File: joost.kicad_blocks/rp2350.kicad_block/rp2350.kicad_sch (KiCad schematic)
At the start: 44 parts, among them U1 GT-USB-7010ASV, U2 RP2350_80QFN, U3 W25Q128, U4 APS6404L-3SQR-SN_C5333729, Y1 ABM8-272-T3

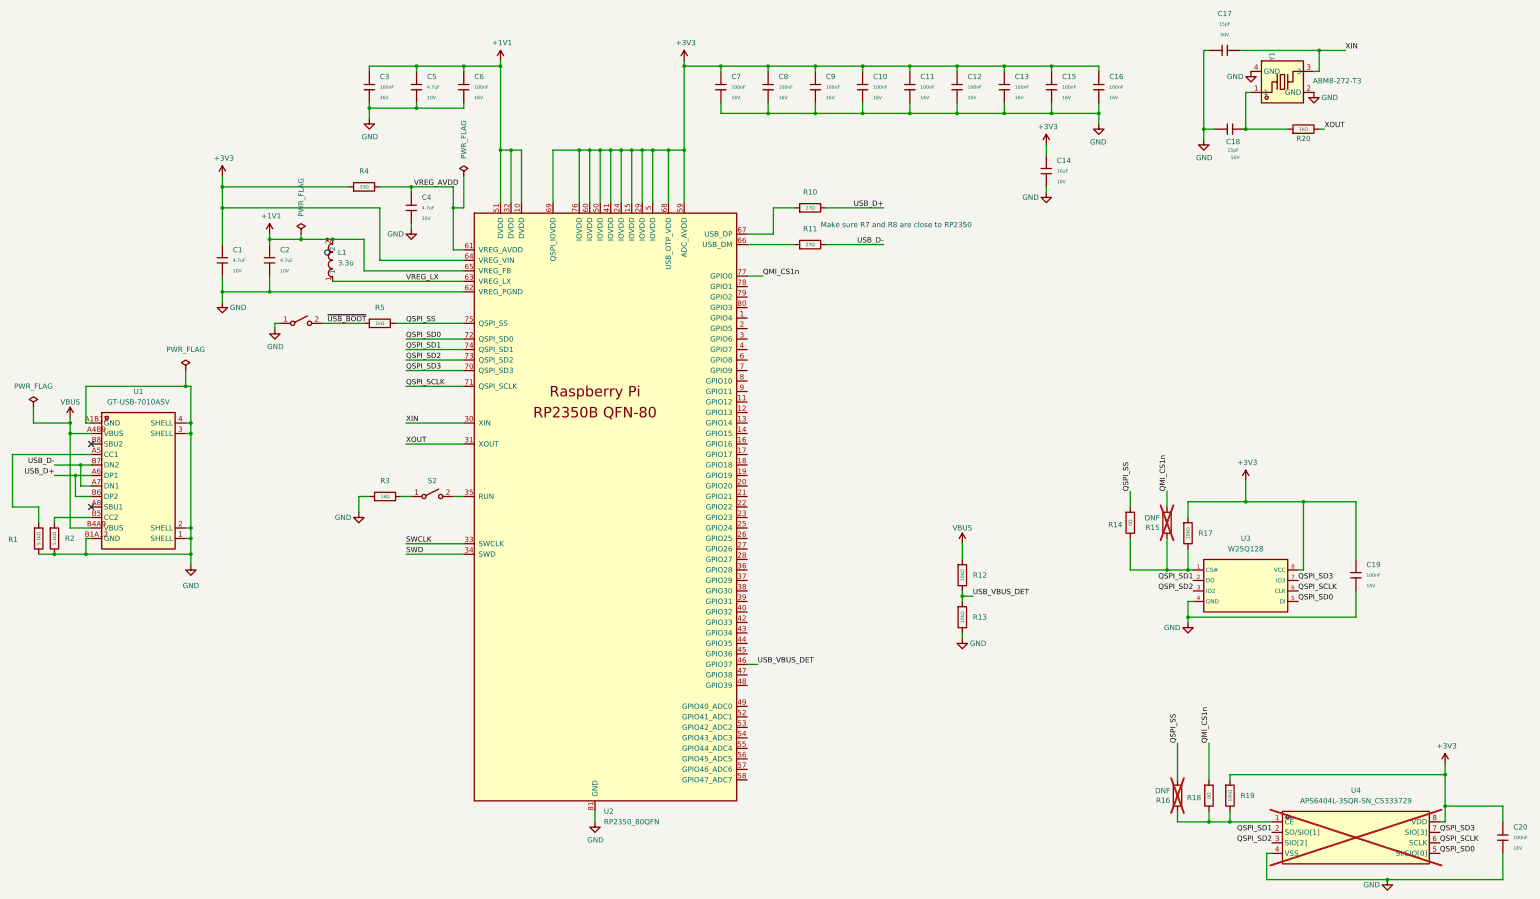
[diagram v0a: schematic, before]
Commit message: -
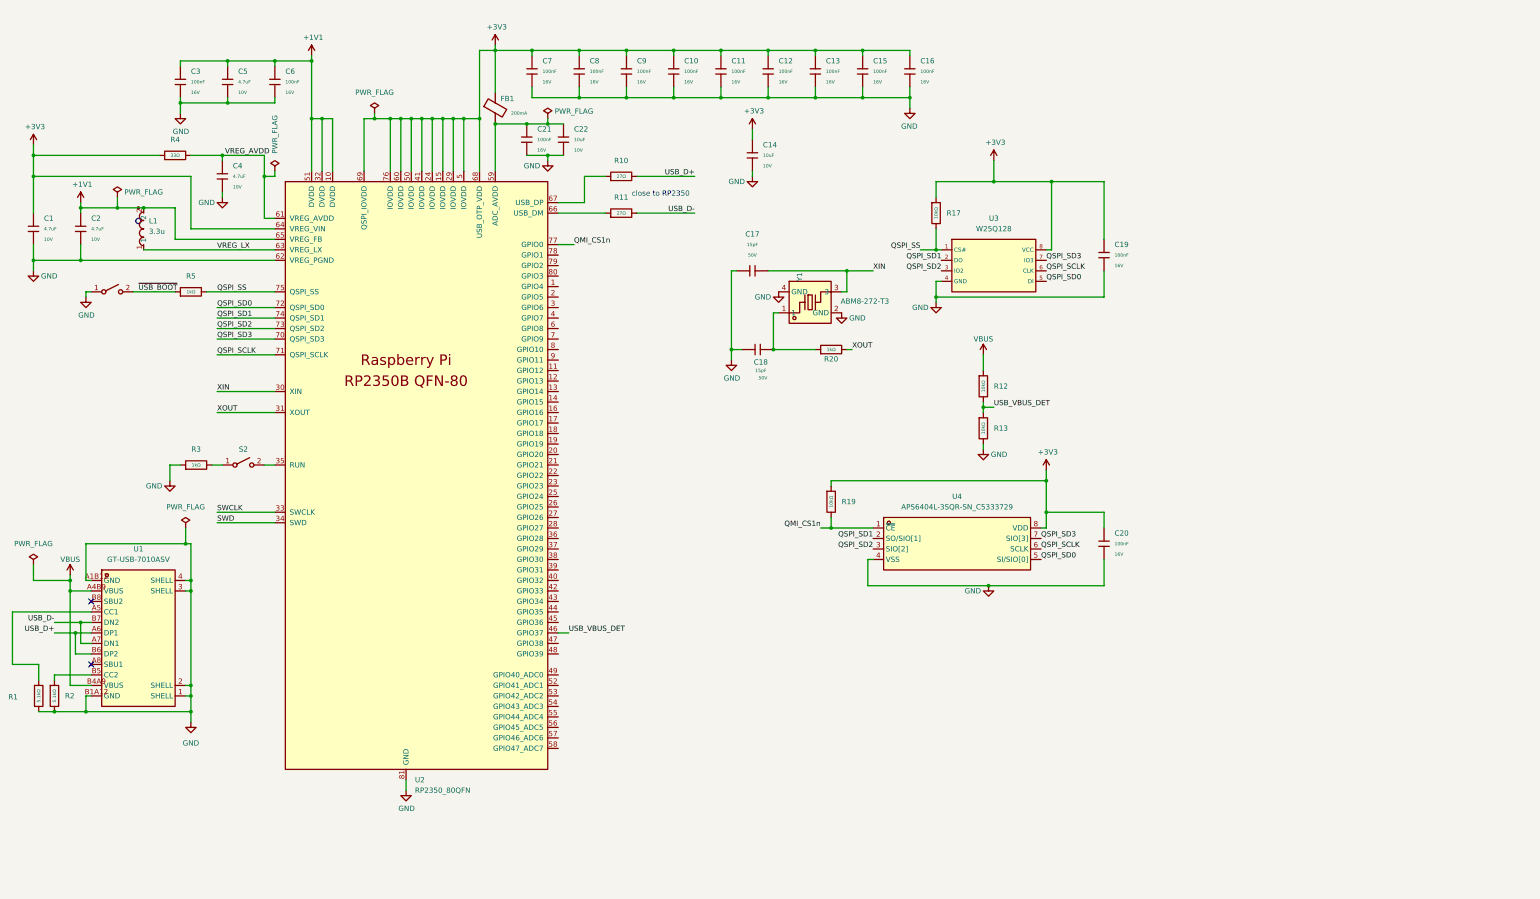
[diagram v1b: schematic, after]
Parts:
- removed R14, R18: 0Ω, PCM_JLCPCB:R_0603, symbol PCM_JLCPCB-Resistors:0603,0Ω
- removed R15, R16: DNF, Resistor_SMD:R_0603_1608Metric, symbol Device:R
- added C21: 100nF, PCM_JLCPCB:C_0402, symbol PCM_JLCPCB-Capacitors:0402,100nF
- added C22: 10uF, PCM_JLCPCB:C_0603, symbol PCM_JLCPCB-Capacitors:0603,10uF
- added FB1: (no value), PCM_JLCPCB:FB_0603, symbol PCM_JLCPCB-Inductors:Ferrite,0603
- U2: symbol projectlibrary:RP2350_80QFN -> joost:RP2350_80QFN
- U4: footprint easyeda2kicad:SOIC-8_L4.9-W3.9-P1.27-LS6.0-BL -> joost:SOIC-8_L4.9-W3.9-P1.27-LS6.0-BL; symbol easyeda2kicad:APS6404L-3SQR-SN_C5333729 -> joost:APS6404L-3SQR-SN_C5333729; now fitted
- Y1: footprint easyeda2kicad:CRYSTAL-SMD_4P-L3.2-W2.5-BL -> joost:CRYSTAL-SMD_4P-L3.2-W2.5-BL; symbol easyeda2kicad:ABM8-272-T3_C20625731 -> joost:ABM8-272-T3_C20625731
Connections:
- net +3V3: now also FB1.1; no longer U2.59 (ADC_AVDD)
- net GND: now also C21.2, C22.2
- net QMI_CS1n: now also R19.2, U4.1 (~{CE})
- net QSPI_SS: now also R17.2, U3.1 (CS#)
- new net: C21.1, C22.1, FB1.2, U2.59 (ADC_AVDD)
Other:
- note added: "close to RP2350"
- note removed: "Make sure R7 and R8 are close to RP2350"
- moved on the sheet: C1, C10, C11, C12, C13, C14, C15, C16, C17, C18, C19, C2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
